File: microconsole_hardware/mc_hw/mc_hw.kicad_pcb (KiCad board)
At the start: 2 copper layers, 6.3 x 6.3 mm, 39 parts, among them SW1 DPAD - UP, SW10 START, SW11 L1, SW12 R1, SW13 L2, SW14 R2, SW16 Joystick, SW17 Joystick, SW2 DPAD - DOWN, SW3 DPAD - LEFT, SW4 DPAD - RIGHT, SW5 A, SW6 B, SW7 X, SW8 Y, SW9 SELECT, U1 ILI9341 / ST7796S SPI LCD, U2 MAX98357A, U3 MCP23017x-x-SO

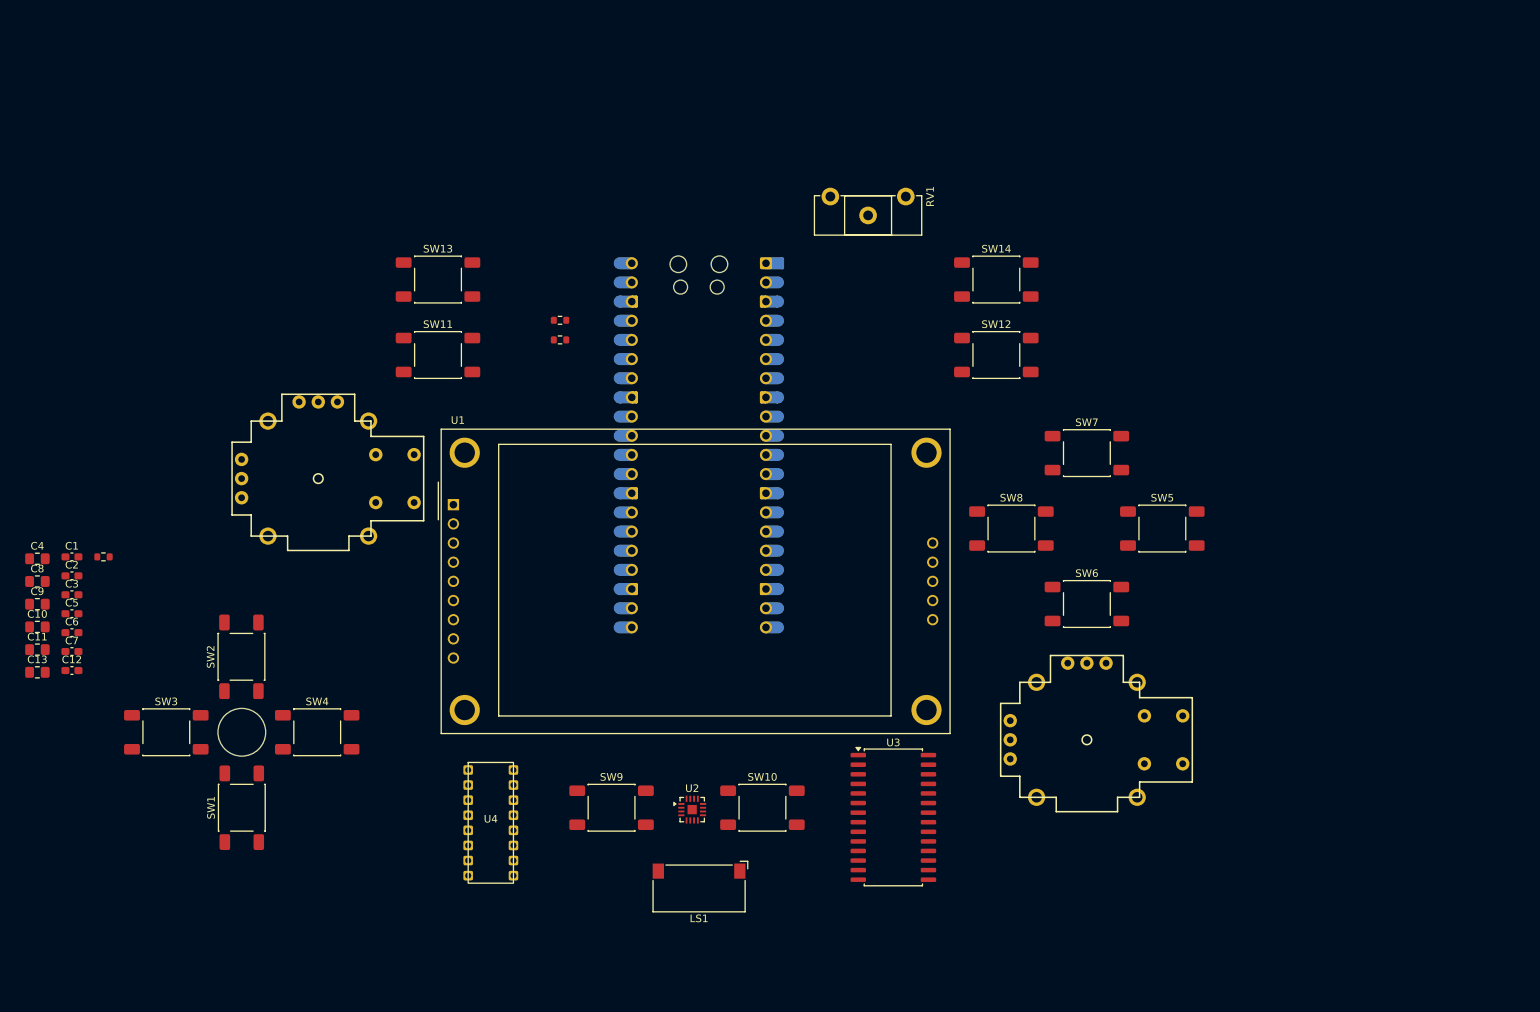
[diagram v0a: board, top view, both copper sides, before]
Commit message: update symbols and libraries
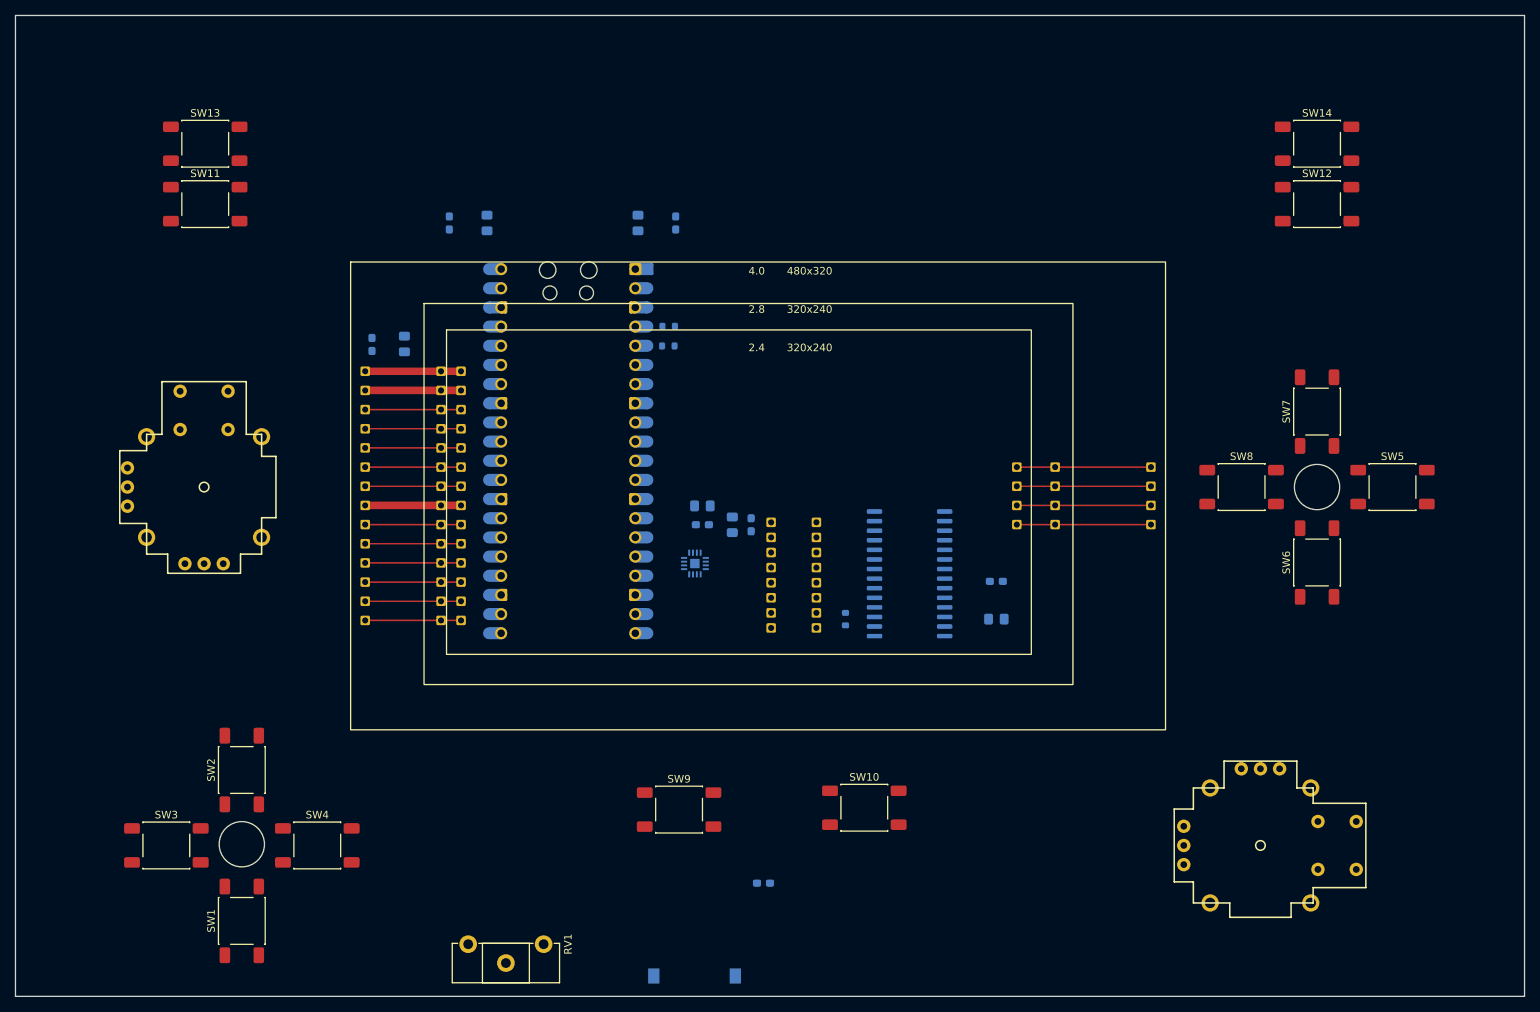
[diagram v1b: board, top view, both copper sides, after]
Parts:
- C1, C10, C11, C12, C13, C2, C3, C4, C5, C6, C7, C8, C9, LS1, R1, R2, R3, U2, U3, U4: moved to B.Cu
- U1: footprint Display:CR2013-MI2120 -> microconsole:TFT
- moved C9 127.1 mm to (180.0, 105.0)
- moved C2 122.5 mm to (180.0, 100.0), turned to 180 degrees
- moved RV1 110.1 mm to (120.0, 148.1)
- moved C1 101.3 mm to (149.1, 140.0), turned to 180 degrees
- moved R3 98.7 mm to (160.0, 105.0), turned to -90 degrees
- moved C11 97.6 mm to (132.5, 52.5), turned to 90 degrees
- moved C6 96.7 mm to (137.5, 52.5), turned to -90 degrees
- moved C4 92.2 mm to (145.0, 92.5), turned to -90 degrees
- moved C7 91.6 mm to (147.5, 92.5), turned to -90 degrees
- moved C8 88.7 mm to (141.0, 90.0)
- moved C13 84.3 mm to (112.5, 52.5), turned to -90 degrees
- moved C3 84.1 mm to (141.0, 92.5)
- moved C12 77.6 mm to (107.5, 52.5), turned to 90 degrees
- moved C10 61.4 mm to (101.5, 68.5), turned to 90 degrees
- moved C5 53.4 mm to (97.2, 68.6), turned to -90 degrees
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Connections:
- C5 pad 1: 3v3 -> VBUS
- U3 pad 4: unconnected-(U3-GPB3-Pad4) -> MCP GPB3 / L1
- U3 pad 5: unconnected-(U3-GPB4-Pad5) -> MCP GPB4 / R1
- U3 pad 6: unconnected-(U3-GPB5-Pad6) -> MCP GPB5 / L2
- U3 pad 7: unconnected-(U3-GPB6-Pad7) -> MCP GPB6 / R2
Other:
- board size 6.3 x 6.3 mm -> 200 x 130 mm

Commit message: update hardware
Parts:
- U1: footprint microconsole:TFT -> microconsole_hardware:TFT
- U4: footprint microconsole:PCB0029_Footprint -> microconsole_hardware:PCB0029_Footprint
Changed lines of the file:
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@@
 		)
 	)
-	(footprint "microconsole:TFT"
+	(footprint "microconsole_hardware:TFT"
 		(layer "F.Cu")
 		(at 147.150001 105.175)
@@
 		(embedded_fonts no)
 		(model "${KICAD10_3DMODEL_DIR}/Display.3dshapes/CR2013-MI2120.step"
-			(hide yes)
 			(offset
 				(xyz 0 0 0)
@@
 			)
 		)
-		(property "Datasheet" "~"
+		(property "Datasheet" ""
 			(at 0 0 90)
 			(layer "B.Fab")
@@
 			)
 		)
-		(property "Description" "100nF volume ADC noise filter"
+		(property "Description" "Unpolarized capacitor"
 			(at 0 0 90)
 			(layer "B.Fab")
@@
 			(roundrect_rratio 0.212766)
 			(net "GND")
-			(pinfunction "~_1")
 			(pintype "passive")
 		)
@@
 			(roundrect_rratio 0.212766)
 			(net "VBUS")
-			(pinfunction "~_2")
 			(pintype "passive")
 		)
@@
 			)
 		)
-		(property "Datasheet" "~"
+		(property "Datasheet" ""
 			(at 0 0 0)
 			(layer "B.Fab")
@@
 			)
 		)
-		(property "Description" "100nF volume ADC noise filter"
+		(property "Description" "Unpolarized capacitor"
 			(at 0 0 0)
 			(layer "B.Fab")
@@
 			(roundrect_rratio 0.212766)
 			(net "GND")
-			(pinfunction "~_1")
 			(pintype "passive")
 		)
@@
 			(roundrect_rratio 0.212766)
 			(net "VBUS")
-			(pinfunction "~_2")
 			(pintype "passive")
 		)
@@
 			)
 		)
-		(property "Datasheet" "~"
+		(property "Datasheet" ""
 			(at 0 0 90)
 			(layer "B.Fab")
@@
 			)
 		)
-		(property "Description" "100nF volume ADC noise filter"
+		(property "Description" "Unpolarized capacitor"
 			(at 0 0 90)
 			(layer "B.Fab")
@@
 			(roundrect_rratio 0.25)
 			(net "3v3")
-			(pinfunction "~_1")
 			(pintype "passive")
 		)
@@
 			(roundrect_rratio 0.25)
 			(net "GND")
-			(pinfunction "~_2")
 			(pintype "passive")
 		)
@@
 			)
 		)
-		(property "Datasheet" "~"
+		(property "Datasheet" ""
 			(at 0 0 0)
 			(layer "B.Fab")
@@
 			)
 		)
-		(property "Description" "100nF volume ADC noise filter"
+		(property "Description" "Unpolarized capacitor"
 			(at 0 0 0)
 			(layer "B.Fab")
@@
 			(roundrect_rratio 0.212766)
 			(net "GND")
-			(pinfunction "~_1")
 			(pintype "passive")
 		)
@@
 			(roundrect_rratio 0.212766)
 			(net "3v3")
-			(pinfunction "~_2")
 			(pintype "passive")
 		)
@@
 			)
 		)
-		(property "Datasheet" "~"
+		(property "Datasheet" ""
 			(at 0 0 90)
 			(layer "B.Fab")
@@
 			)
 		)
-		(property "Description" "100nF volume ADC noise filter"
+		(property "Description" "Unpolarized capacitor"
 			(at 0 0 90)
 			(layer "B.Fab")
@@
 			(roundrect_rratio 0.212766)
 			(net "GND")
-			(pinfunction "~_1")
 			(pintype "passive")
 		)
@@
 			(roundrect_rratio 0.212766)
 			(net "3v3")
-			(pinfunction "~_2")
 			(pintype "passive")
 		)
@@
 			)
 		)
-		(property "Datasheet" "~"
+		(property "Datasheet" ""
 			(at 0 0 0)
 			(layer "B.Fab")
@@
 			)
 		)
-		(property "Description" "100nF volume ADC noise filter"
+		(property "Description" "Unpolarized capacitor"
 			(at 0 0 0)
 			(layer "B.Fab")
@@
 			(roundrect_rratio 0.25)
 			(net "3v3")
-			(pinfunction "~_1")
 			(pintype "passive")
 		)
@@
 			(roundrect_rratio 0.25)
 			(net "GND")
-			(pinfunction "~_2")
 			(pintype "passive")
 		)
@@
 			)
 		)
-		(property "Datasheet" "~"
+		(property "Datasheet" ""
 			(at 0 0 90)
 			(layer "B.Fab")
@@
 			)
 		)
-		(property "Description" "100nF volume ADC noise filter"
+		(property "Description" "Unpolarized capacitor"
 			(at 0 0 90)
 			(layer "B.Fab")
@@
 			(roundrect_rratio 0.25)
 			(net "VBUS")
-			(pinfunction "~_1")
 			(pintype "passive")
 		)
@@
 			(roundrect_rratio 0.25)
 			(net "GND")
-			(pinfunction "~_2")
 			(pintype "passive")
 		)
@@
 			)
 		)
-		(property "Datasheet" "~"
+		(property "Datasheet" ""
 			(at 0 0 90)
 			(layer "B.Fab")
@@
 			)
 		)
-		(property "Description" "100nF volume ADC noise filter"
+		(property "Description" "Unpolarized capacitor"
 			(at 0 0 90)
 			(layer "B.Fab")
@@
 			(roundrect_rratio 0.25)
 			(net "GND")
-			(pinfunction "~_1")
 			(pintype "passive")
 		)
@@
 			(roundrect_rratio 0.25)
 			(net "VBUS")
-			(pinfunction "~_2")
 			(pintype "passive")
 		)
@@
 			)
 		)
-		(property "Datasheet" "~"
+		(property "Datasheet" ""
 			(at 0 0 90)
 			(layer "B.Fab")
@@
 			)
 		)
-		(property "Description" "100nF volume ADC noise filter"
+		(property "Description" "Unpolarized capacitor"
 			(at 0 0 90)
 			(layer "B.Fab")
@@
 			(roundrect_rratio 0.25)
 			(net "VBUS")
-			(pinfunction "~_1")
 			(pintype "passive")
 		)
@@
 			(roundrect_rratio 0.25)
 			(net "GND")
-			(pinfunction "~_2")
 			(pintype "passive")
 		)
@@
 			)
 		)
-		(property "Datasheet" "~"
+		(property "Datasheet" ""
 			(at 0 0 0)
 			(layer "B.Fab")
@@
 			)
 		)
-		(property "Description" "100nF volume ADC noise filter"
+		(property "Description" "Unpolarized capacitor"
 			(at 0 0 0)
 			(layer "B.Fab")
@@
 			(roundrect_rratio 0.25)
 			(net "AGND")
-			(pinfunction "~_1")
 			(pintype "passive")
 		)
@@
 			(roundrect_rratio 0.25)
 			(net "GPIO28 {slash} VOLUME POT")
-			(pinfunction "~_2")
 			(pintype "passive")
 		)
@@
 			(net "GND")
 			(pinfunction "PAD_17")
-			(pintype "unspecified")
+			(pintype "power_in")
 			(zone_connect 2)
 		)
@@
 			(roundrect_rratio 0.25)
 			(net "GPIO3 {slash} MCP|ADC SCL")
-			(pinfunction "SCL_12")
+			(pinfunction "SCK_12")
 			(pintype "input")
 		)
@@
 			)
 		)
-		(property "Datasheet" "~"
+		(property "Datasheet" ""
 			(at 0 0 90)
 			(layer "B.Fab")
@@
 			)
 		)
-		(property "Description" "100nF volume ADC noise filter"
+		(property "Description" "Unpolarized capacitor"
 			(at 0 0 90)
 			(layer "B.Fab")
@@
 			(roundrect_rratio 0.212766)
 			(net "GND")
-			(pinfunction "~_1")
 			(pintype "passive")
 		)
@@
 			(roundrect_rratio 0.212766)
 			(net "VBUS")
-			(pinfunction "~_2")
 			(pintype "passive")
 		)
@@
 			)
 		)
-		(property "Datasheet" "~"
+		(property "Datasheet" ""
 			(at 0 0 0)
 			(layer "B.Fab")
@@
 			)
 		)
-		(property "Description" "100nF volume ADC noise filter"
+		(property "Description" "Unpolarized capacitor"
 			(at 0 0 0)
 			(layer "B.Fab")
@@
 			(roundrect_rratio 0.25)
 			(net "GND")
-			(pinfunction "~_1")
 			(pintype "passive")
 		)
@@
 			(roundrect_rratio 0.25)
 			(net "VBUS")
-			(pinfunction "~_2")
 			(pintype "passive")
 		)
@@
 		)
 	)
-	(footprint "microconsole:PCB0029_Footprint"
+	(footprint "microconsole_hardware:PCB0029_Footprint"
 		(layer "B.Cu")
 		(at 153.150001 99.175 180)
@@
 			)
 		)
-		(property "Datasheet" "~"
+		(property "Datasheet" ""
 			(at 0 0 90)
 			(layer "B.Fab")
@@
 			)
 		)
-		(property "Description" "100nF volume ADC noise filter"
+		(property "Description" "Unpolarized capacitor"
 			(at 0 0 90)
 			(layer "B.Fab")
@@
 			(roundrect_rratio 0.212766)
 			(net "GND")
-			(pinfunction "~_1")
 			(pintype "passive")
 		)
@@
 			(roundrect_rratio 0.212766)
 			(net "VBUS")
-			(pinfunction "~_2")
 			(pintype "passive")
 		)
